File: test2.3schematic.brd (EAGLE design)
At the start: 17.5 x 30 mm, 29 parts, among them IC1 NCS21911SN2T1G, IC2 FXLN8371QR1, IC3 MAX25210ATAB9_V+, IC4 NCS21911SN2T1G, IC5 NCS21911SN2T1G

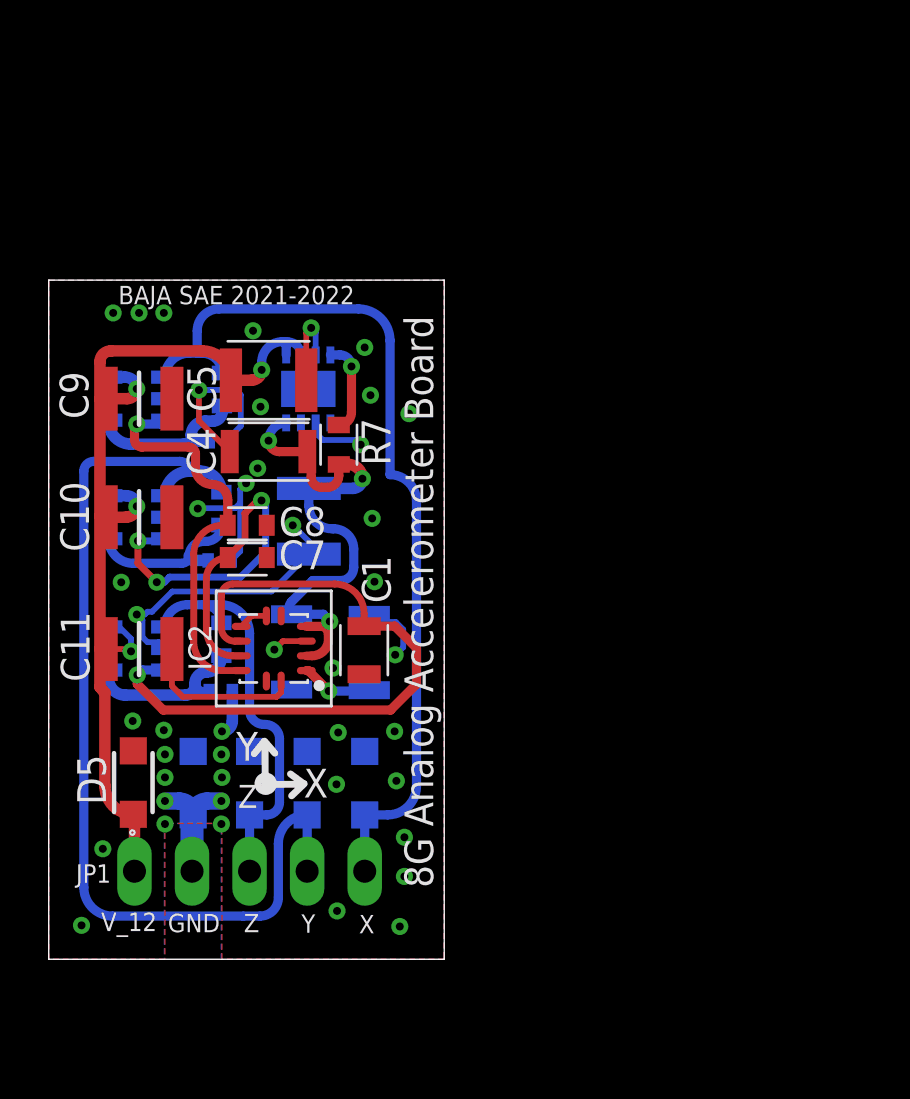
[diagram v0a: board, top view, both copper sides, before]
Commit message: Added Advance circuits logo and gerber file
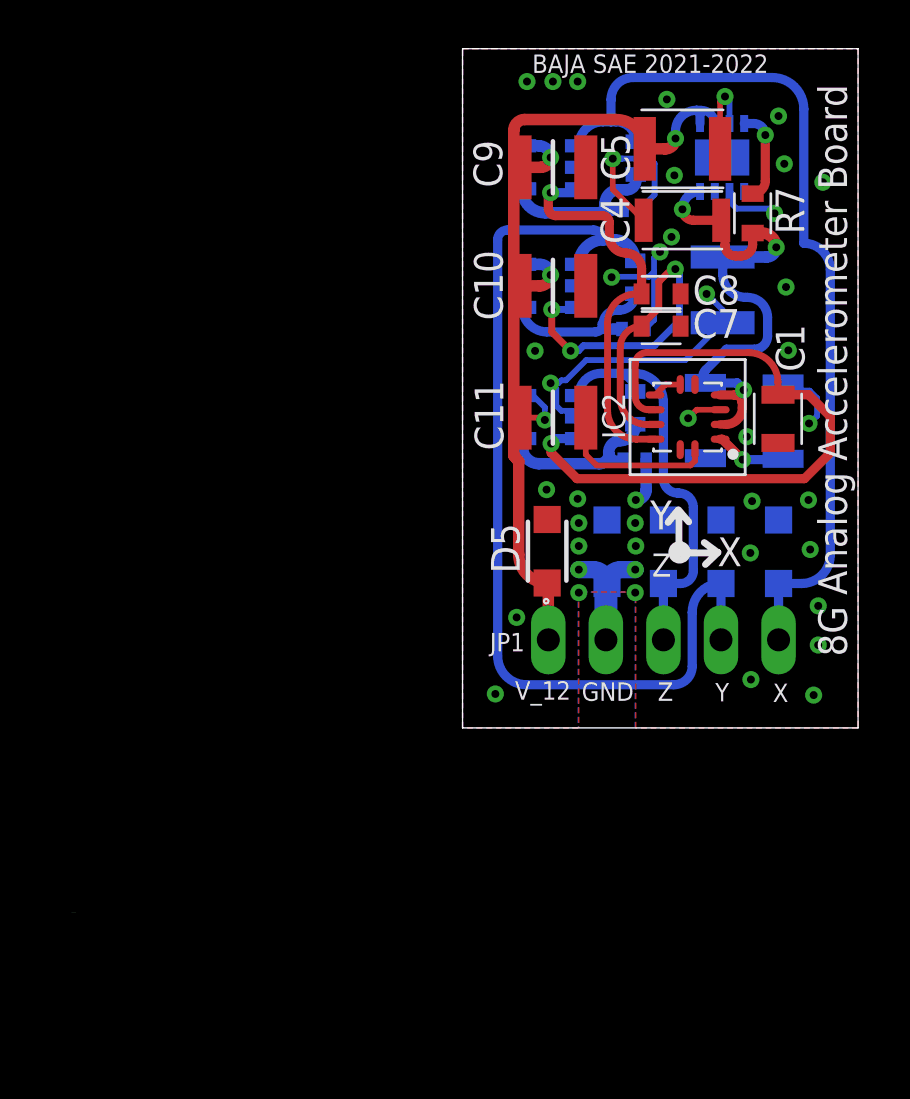
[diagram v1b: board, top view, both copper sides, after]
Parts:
- moved C10 20.9 mm to (21.3, 27.6)
- moved C9 20.9 mm to (21.3, 32.9)
- moved D3 20.9 mm to (26.1, 15.9)
- moved IC1 20.9 mm to (21.2, 32.9)
- moved IC4 20.9 mm to (21.2, 27.6)
- moved JP1 20.9 mm to (26.1, 12.0)
- moved R5 20.9 mm to (24.9, 28.0)
- moved R6 20.9 mm to (24.9, 33.3)
- moved C1 20.9 mm to (31.2, 21.8)
- moved C11 20.9 mm to (21.3, 21.8)
- moved C2 20.9 mm to (28.8, 27.5)
- moved C3 20.9 mm to (28.0, 21.7)
- moved C4 20.9 mm to (27.0, 30.5)
- moved C5 20.9 mm to (27.0, 33.7)
- moved C6 20.9 mm to (31.4, 21.7)
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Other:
- board text added: "C:/Users/forre/Downloads/adv.bmp"
